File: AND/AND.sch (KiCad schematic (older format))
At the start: 2 parts

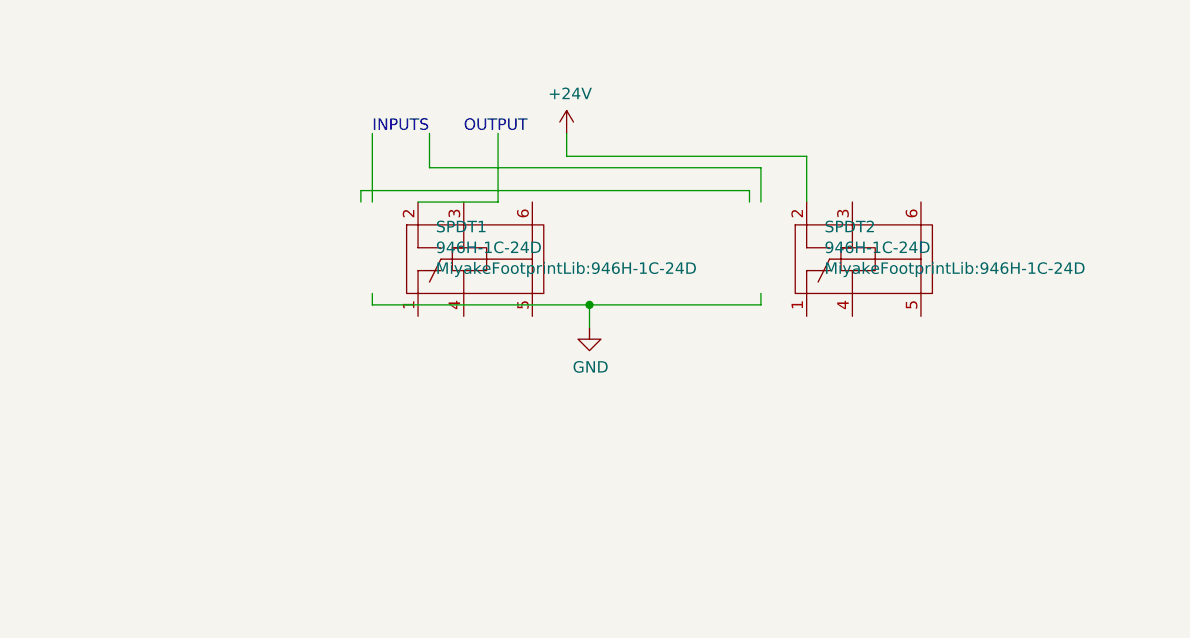
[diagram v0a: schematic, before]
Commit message: Add files via upload
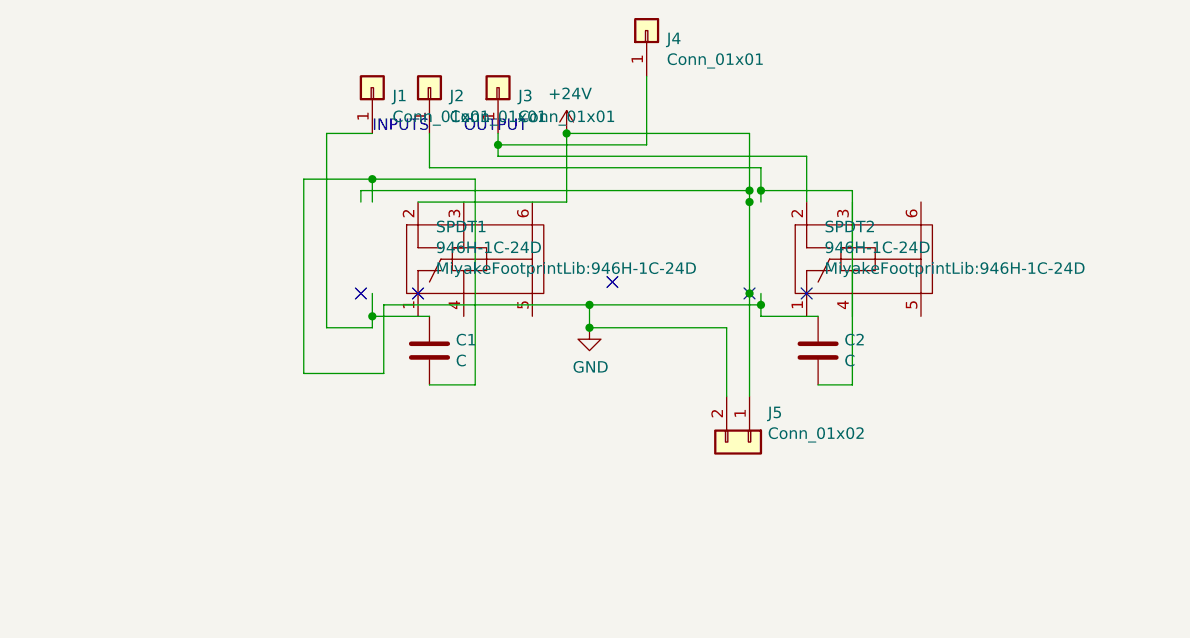
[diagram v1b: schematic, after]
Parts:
- added C1, C2: C, MiyakeFootprintLib:Condensor, symbol Device:C
- added J1, J2, J3, J4: Conn_01x01, Connector_PinHeader_2.54mm:PinHeader_1x01_P2.54mm_Vertical, symbol Connector_Generic:Conn_01x01
- added J5: Conn_01x02, Connector_PinHeader_2.54mm:PinHeader_1x02_P2.54mm_Vertical, symbol Connector_Generic:Conn_01x02
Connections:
- wire segments 17 -> 44
- no-connect marks 0 -> 5
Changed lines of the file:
@@
 $EndDescr
+$Comp
+L MiyakeLib:946H-1C-24D SPDT2
+U 1 1 5ED25E6C
+P 5450 3050
+F 0 "SPDT2" V 5541 2822 50  0000 R CNN
+F 1 "946H-1C-24D" V 5450 2822 50  0000 R CNN
+F 2 "MiyakeFootprintLib:946H-1C-24D" V 5359 2822 50  0000 R CNN
+F 3 "" H 5400 3300 50  0001 C CNN
+	1    5450 3050
+	0    -1   -1   0
+$EndComp
+Wire Wire Line
+	5350 2800 3650 2800
+Wire Wire Line
+	3650 2800 3650 2850
+Wire Wire Line
+	5400 2850 5400 2800
+Wire Wire Line
+	5400 2700 3950 2700
+Wire Wire Line
+	3950 2700 3950 2550
+Wire Wire Line
+	5400 3250 5400 3300
+Wire Wire Line
+	5400 3300 4650 3300
+Wire Wire Line
+	4650 3300 4650 3400
+Text Notes 3700 2550 0    50   ~ 0
+INPUTS
+Text Notes 4100 2550 0    50   ~ 0
+OUTPUT
+$Comp
+L power:+24V #PWR01
+U 1 1 5ED293DD
+P 4550 2550
+F 0 "#PWR01" H 4550 2400 50  0001 C CNN
+F 1 "+24V" H 4565 2723 50  0000 C CNN
+F 2 "" H 4550 2550 50  0001 C CNN
+F 3 "" H 4550 2550 50  0001 C CNN
+	1    4550 2550
+	1    0    0    -1
+$EndComp
+$Comp
+L power:GND #PWR02
+U 1 1 5ED29766
+P 4650 3400
+F 0 "#PWR02" H 4650 3150 50  0001 C CNN
+F 1 "GND" H 4655 3227 50  0000 C CNN
+F 2 "" H 4650 3400 50  0001 C CNN
+F 3 "" H 4650 3400 50  0001 C CNN
+	1    4650 3400
+	1    0    0    -1
+$EndComp
+$Comp
+L Connector_Generic:Conn_01x01 J1
+U 1 1 5ED5987F
+P 3700 2350
+F 0 "J1" V 3664 2262 50  0000 R CNN
+F 1 "Conn_01x01" V 3573 2262 50  0000 R CNN
+F 2 "Connector_PinHeader_2.54mm:PinHeader_1x01_P2.54mm_Vertical" H 3700 2350 50  0001 C CNN
+F 3 "~" H 3700 2350 50  0001 C CNN
+	1    3700 2350
+	0    -1   -1   0
+$EndComp
+$Comp
+L Connector_Generic:Conn_01x01 J2
+U 1 1 5ED59E15
+P 3950 2350
+F 0 "J2" V 3914 2262 50  0000 R CNN
+F 1 "Conn_01x01" V 3823 2262 50  0000 R CNN
+F 2 "Connector_PinHeader_2.54mm:PinHeader_1x01_P2.54mm_Vertical" H 3950 2350 50  0001 C CNN
+F 3 "~" H 3950 2350 50  0001 C CNN
+	1    3950 2350
+	0    -1   -1   0
+$EndComp
+$Comp
+L Connector_Generic:Conn_01x01 J3
+U 1 1 5ED5A11E
+P 4250 2350
+F 0 "J3" V 4214 2262 50  0000 R CNN
+F 1 "Conn_01x01" V 4123 2262 50  0000 R CNN
+F 2 "Connector_PinHeader_2.54mm:PinHeader_1x01_P2.54mm_Vertical" H 4250 2350 50  0001 C CNN
+F 3 "~" H 4250 2350 50  0001 C CNN
+	1    4250 2350
+	0    -1   -1   0
+$EndComp
+NoConn ~ 3650 3250
+NoConn ~ 5350 3250
+NoConn ~ 5600 3250
+NoConn ~ 4750 3200
+Wire Wire Line
+	4250 2600 4900 2600
+Wire Wire Line
+	4900 2600 4900 2300
+Connection ~ 4250 2600
+Wire Wire Line
+	4250 2600 4250 2550
+$Comp
+L Connector_Generic:Conn_01x01 J4
+U 1 1 5ED5C648
+P 4900 2100
+F 0 "J4" V 4864 2012 50  0000 R CNN
+F 1 "Conn_01x01" V 4773 2012 50  0000 R CNN
+F 2 "Connector_PinHeader_2.54mm:PinHeader_1x01_P2.54mm_Vertical" H 4900 2100 50  0001 C CNN
+F 3 "~" H 4900 2100 50  0001 C CNN
+	1    4900 2100
+	0    -1   -1   0
+$EndComp
+Connection ~ 4650 3400
+Wire Wire Line
+	4550 2550 5350 2550
+Wire Wire Line
+	5350 2550 5350 2800
+Connection ~ 5350 2800
+Wire Wire Line
+	5350 2800 5350 2850
+Connection ~ 5350 2850
+Wire Wire Line
+	5350 2850 5350 3250
+Connection ~ 5350 3250
+Wire Wire Line
+	5250 3400 5250 3700
+Wire Wire Line
+	4650 3400 5250 3400
+$Comp
+L Connector_Generic:Conn_01x02 J5
+U 1 1 5ED5FF3D
+P 5350 3900
+F 0 "J5" V 5222 3980 50  0000 L CNN
+F 1 "Conn_01x02" V 5313 3980 50  0000 L CNN
+F 2 "Connector_PinHeader_2.54mm:PinHeader_1x02_P2.54mm_Vertical" H 5350 3900 50  0001 C CNN
+F 3 "~" H 5350 3900 50  0001 C CNN
+	1    5350 3900
+	0    1    1    0
+$EndComp
+Wire Wire Line
+	3700 2550 3500 2550
+Wire Wire Line
+	3500 2550 3500 3400
+Wire Wire Line
+	3500 3400 3700 3400
+Wire Wire Line
+	3750 3300 3750 3600
+Wire Wire Line
+	3750 3600 3400 3600
+Wire Wire Line
+	3400 3600 3400 2750
+Wire Wire Line
+	3400 2750 3700 2750
+Wire Wire Line
+	3700 2750 3700 2850
+Connection ~ 4650 3300
+Wire Wire Line
+	4650 3300 3750 3300
+NoConn ~ 3900 3250
 $Comp
 L MiyakeLib:946H-1C-24D SPDT1
@@
 	0    -1   -1   0
 $EndComp
-$Comp
-L MiyakeLib:946H-1C-24D SPDT2
-U 1 1 5ED25E6C
-P 5450 3050
-F 0 "SPDT2" V 5541 2822 50  0000 R CNN
-F 1 "946H-1C-24D" V 5450 2822 50  0000 R CNN
-F 2 "MiyakeFootprintLib:946H-1C-24D" V 5359 2822 50  0000 R CNN
-F 3 "" H 5400 3300 50  0001 C CNN
-	1    5450 3050
-	0    -1   -1   0
-$EndComp
-Wire Wire Line
-	5350 2850 5350 2800
-Wire Wire Line
-	5350 2800 3650 2800
-Wire Wire Line
-	3650 2800 3650 2850
-Wire Wire Line
-	3700 2850 3700 2550
-Wire Wire Line
-	5400 2850 5400 2700
-Wire Wire Line
-	5400 2700 3950 2700
-Wire Wire Line
-	3950 2700 3950 2550
-Wire Wire Line
-	3900 2850 4250 2850
-Wire Wire Line
-	4250 2850 4250 2550
 Wire Wire Line
 	5600 2850 5600 2650
 Wire Wire Line
-	5600 2650 4550 2650
-Wire Wire Line
-	4550 2650 4550 2550
-Wire Wire Line
-	5400 3250 5400 3300
-Wire Wire Line
-	5400 3300 4650 3300
-Wire Wire Line
-	3700 3300 3700 3250
-Wire Wire Line
-	4650 3300 4650 3400
-Connection ~ 4650 3300
-Wire Wire Line
-	4650 3300 3700 3300
-Text Notes 3700 2550 0    50   ~ 0
-INPUTS
-Text Notes 4100 2550 0    50   ~ 0
-OUTPUT
-$Comp
-L power:+24V #PWR01
-U 1 1 5ED293DD
-P 4550 2550
-F 0 "#PWR01" H 4550 2400 50  0001 C CNN
-F 1 "+24V" H 4565 2723 50  0000 C CNN
-F 2 "" H 4550 2550 50  0001 C CNN
-F 3 "" H 4550 2550 50  0001 C CNN
-	1    4550 2550
-	1    0    0    -1
-$EndComp
-$Comp
-L power:GND #PWR02
-U 1 1 5ED29766
-P 4650 3400
-F 0 "#PWR02" H 4650 3150 50  0001 C CNN
-F 1 "GND" H 4655 3227 50  0000 C CNN
-F 2 "" H 4650 3400 50  0001 C CNN
-F 3 "" H 4650 3400 50  0001 C CNN
-	1    4650 3400
-	1    0    0    -1
-$EndComp
+	5600 2650 4250 2650
+Wire Wire Line
+	4250 2650 4250 2600
+Wire Wire Line
+	3900 2850 4550 2850
+Wire Wire Line
+	4550 2850 4550 2550
+Connection ~ 4550 2550
+$Comp
+L Device:C C2
+U 1 1 5ED6B58C
+P 5650 3500
+F 0 "C2" H 5765 3546 50  0000 L CNN
+F 1 "C" H 5765 3455 50  0000 L CNN
+F 2 "MiyakeFootprintLib:Condensor" H 5688 3350 50  0001 C CNN
+F 3 "~" H 5650 3500 50  0001 C CNN
+	1    5650 3500
+	1    0    0    -1
+$EndComp
+$Comp
+L Device:C C1
+U 1 1 5ED6C491
+P 3950 3500
+F 0 "C1" H 4065 3546 50  0000 L CNN
+F 1 "C" H 4065 3455 50  0000 L CNN
+F 2 "MiyakeFootprintLib:Condensor" H 3988 3350 50  0001 C CNN
+F 3 "~" H 3950 3500 50  0001 C CNN
+	1    3950 3500
+	1    0    0    -1
+$EndComp
+Wire Wire Line
+	3700 3250 3700 3350
+Wire Wire Line
+	5350 3250 5350 3700
+Wire Wire Line
+	5650 3350 5400 3350
+Wire Wire Line
+	5400 3350 5400 3300
+Connection ~ 5400 3300
+Wire Wire Line
+	5650 3650 5800 3650
+Wire Wire Line
+	5800 3650 5800 2800
+Wire Wire Line
+	5800 2800 5400 2800
+Connection ~ 5400 2800
+Wire Wire Line
+	5400 2800 5400 2700
+Wire Wire Line
+	3950 3350 3700 3350
+Connection ~ 3700 3350
+Wire Wire Line
+	3700 3350 3700 3400
+Wire Wire Line
+	3950 3650 4150 3650
+Wire Wire Line
+	4150 3650 4150 2750
+Wire Wire Line
+	4150 2750 3700 2750
+Connection ~ 3700 2750
 $EndSCHEMATC

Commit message: Add files via upload
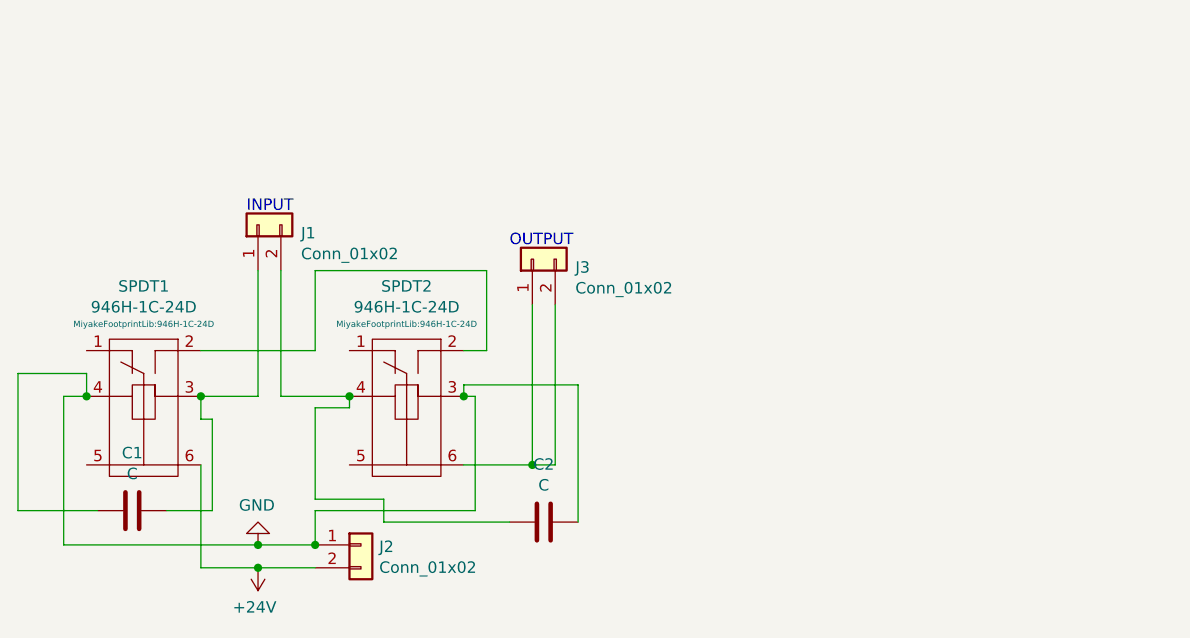
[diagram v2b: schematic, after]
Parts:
- removed J1, J2, J3, J4: Conn_01x01, Connector_PinHeader_2.54mm:PinHeader_1x01_P2.54mm_Vertical, symbol Connector_Generic:Conn_01x01
- removed J5: Conn_01x02, Connector_PinHeader_2.54mm:PinHeader_1x02_P2.54mm_Vertical, symbol Connector_Generic:Conn_01x02
- added J1, J2, J3: Conn_01x02, Connector_PinHeader_2.54mm:PinHeader_1x02_P2.54mm_Vertical, symbol Connector_Generic:Conn_01x02
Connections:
- wire segments 44 -> 41
- no-connect marks 5 -> 0
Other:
- note added: "INPUT"
- note removed: "INPUTS"
